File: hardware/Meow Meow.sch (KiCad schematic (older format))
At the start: 28 parts, among them P1 D, P10 A, P11 W, P12 MOUSE_LEFT, P13 CONN_01X06, P14 CONN_01X06, P2 SPACE, P3 KEY_RIGHT_ARROW, P4 SWD, P5 KEY_LEFT_ARROW, P6 KEY_DOWN_ARROW, P7 KEY_UP_ARROW, P8 S, P9 USB_Micro, SW1 SW_Push, U1 ATSAMD21G18A-AU, U2 AP2114-3.3K

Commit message: Add pin 5v
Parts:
- removed P13, P14: CONN_01X06, Pines:61000618321, symbol CONN_01X06
- added P? (x2): CONN_01X07, symbol CONN_01X07
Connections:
- wire segments 97 -> 101
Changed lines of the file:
@@
 Title "Meow Meow"
 Date "2018-05-16"
-Rev "0.7"
+Rev "0.8"
 Comp "Electronic Cats"
 Comment1 "Andres Sabas"
@@
 	8745 3600 8745 3570
 $Comp
-L CONN_01X06 P13
-U 1 1 5B1DE3E8
-P 9090 6010
-F 0 "P13" H 9090 6360 50  0000 C CNN
-F 1 "CONN_01X06" V 9190 6010 50  0000 C CNN
-F 2 "Pines:61000618321" H 9090 6010 50  0001 C CNN
-F 3 "" H 9090 6010 50  0000 C CNN
-	1    9090 6010
-	1    0    0    -1
-$EndComp
-$Comp
-L CONN_01X06 P14
-U 1 1 5B1DE934
-P 9570 5980
-F 0 "P14" H 9570 6330 50  0000 C CNN
-F 1 "CONN_01X06" V 9670 5980 50  0000 C CNN
-F 2 "Pines:61000618321" H 9570 5980 50  0001 C CNN
-F 3 "" H 9570 5980 50  0000 C CNN
-	1    9570 5980
+L CONN_01X07 P?
+U 1 1 5B26BBAC
+P 9090 6060
+F 0 "P?" H 9090 6460 50  0000 C CNN
+F 1 "CONN_01X07" V 9190 6060 50  0000 C CNN
+F 2 "" H 9090 6060 50  0000 C CNN
+F 3 "" H 9090 6060 50  0000 C CNN
+	1    9090 6060
+	1    0    0    -1
+$EndComp
+$Comp
+L CONN_01X07 P?
+U 1 1 5B26BCF3
+P 9570 6030
+F 0 "P?" H 9570 6430 50  0000 C CNN
+F 1 "CONN_01X07" V 9670 6030 50  0000 C CNN
+F 2 "" H 9570 6030 50  0000 C CNN
+F 3 "" H 9570 6030 50  0000 C CNN
+	1    9570 6030
 	-1   0    0    1
 $EndComp
+Wire Wire Line
+	8355 6360 8890 6360
+$Comp
+L VCC #PWR?
+U 1 1 5B26C1A1
+P 8355 6340
+F 0 "#PWR?" H 8355 6190 50  0001 C CNN
+F 1 "VCC" H 8355 6490 50  0000 C CNN
+F 2 "" H 8355 6340 50  0000 C CNN
+F 3 "" H 8355 6340 50  0000 C CNN
+	1    8355 6340
+	1    0    0    -1
+$EndComp
+Wire Wire Line
+	8355 6360 8355 6340
+Wire Wire Line
+	9770 6330 9815 6330
+Wire Wire Line
+	9815 6330 9815 6230
+Connection ~ 9815 6230
 $EndSCHEMATC

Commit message: connector 6 pin
se quito 3V
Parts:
- removed P? (x2): CONN_01X07, symbol CONN_01X07
- added J? (x2): Conn_02x03_Top_Bottom, symbol Conn_02x03_Top_Bottom
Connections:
- wire segments 101 -> 97
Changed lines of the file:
@@
 Text Notes 7805 5625 0    60   ~ 0
 PIN EXTRAS
-Text Label 9870 5730 0    60   ~ 0
+Text Label 10025 6130 0    60   ~ 0
 I2S_SCK
-Text Label 9875 5830 0    60   ~ 0
+Text Label 10025 6030 0    60   ~ 0
 I2S_D1/X7
-Text Label 9875 5930 0    60   ~ 0
+Text Label 10020 5930 0    60   ~ 0
 TX/X2
-Text Label 9875 6030 0    60   ~ 0
+Text Label 9340 6130 2    60   ~ 0
 RX/X3
-Text Label 8780 5760 2    60   ~ 0
-MOSI
-Text Label 8780 5860 2    60   ~ 0
+Text Label 8105 6025 2    60   ~ 0
 MISO
-Text Label 8780 5960 2    60   ~ 0
+Text Label 8105 6125 2    60   ~ 0
 SCK
-Text Label 9875 6130 0    60   ~ 0
+Text Label 9335 6030 2    60   ~ 0
 CS
-Text Label 8785 6060 2    60   ~ 0
+Text Label 8820 5925 0    60   ~ 0
 SDA
-Text Label 8785 6160 2    60   ~ 0
+Text Label 8815 6025 0    60   ~ 0
 SCL
 $Comp
 L GND #PWR019
 U 1 1 5AFF5159
-P 9890 6230
-F 0 "#PWR019" H 9890 5980 50  0001 C CNN
-F 1 "GND" H 9890 6080 50  0000 C CNN
-F 2 "" H 9890 6230 50  0000 C CNN
-F 3 "" H 9890 6230 50  0000 C CNN
-	1    9890 6230
-	1    0    0    -1
-$EndComp
-$Comp
-L +3.3V #PWR020
-U 1 1 5AFF522D
-P 8500 6260
-F 0 "#PWR020" H 8500 6110 50  0001 C CNN
-F 1 "+3.3V" H 8500 6400 50  0000 C CNN
-F 2 "" H 8500 6260 50  0000 C CNN
-F 3 "" H 8500 6260 50  0000 C CNN
-	1    8500 6260
-	1    0    0    -1
+P 9335 5930
+F 0 "#PWR019" H 9335 5680 50  0001 C CNN
+F 1 "GND" H 9335 5780 50  0000 C CNN
+F 2 "" H 9335 5930 50  0000 C CNN
+F 3 "" H 9335 5930 50  0000 C CNN
+	1    9335 5930
+	-1   0    0    1
 $EndComp
 $Comp
@@
 	3895 1655 4210 1655
 Wire Wire Line
-	3990 1955 3990 1565
-Wire Wire Line
-	3895 1955 3990 1955
+	3990 1565 3990 1955
+Wire Wire Line
+	3990 1955 3895 1955
 Wire Wire Line
 	3945 2285 3945 2340
@@
 Connection ~ 4025 4655
 Wire Wire Line
-	3895 4655 4025 4655
+	4025 4655 3895 4655
 Connection ~ 4025 4555
 Wire Wire Line
-	3895 4555 4025 4555
+	4025 4555 3895 4555
 Wire Wire Line
 	4025 4355 4025 4740
@@
 Connection ~ 9605 1290
 Wire Wire Line
-	9605 1355 9605 1290
+	9605 1290 9605 1355
 Connection ~ 9370 1290
 Wire Wire Line
@@
 	7590 1290 7590 1175
 Wire Wire Line
-	8315 1290 7590 1290
+	7590 1290 8315 1290
 Wire Wire Line
 	9810 5100 9810 5325
@@
 	1590 1655 1590 1675
 Wire Wire Line
-	8890 6160 8785 6160
-Wire Wire Line
-	8890 6060 8785 6060
-Wire Wire Line
-	8890 5960 8780 5960
-Wire Wire Line
-	8890 5860 8780 5860
-Wire Wire Line
-	8890 5760 8780 5760
-Wire Wire Line
-	9770 6130 9875 6130
-Wire Wire Line
-	9770 6030 9875 6030
-Wire Wire Line
-	9770 5930 9875 5930
-Wire Wire Line
-	9770 5830 9875 5830
-Wire Wire Line
-	9770 5730 9870 5730
-Wire Wire Line
-	8500 6260 8890 6260
-Wire Wire Line
-	9770 6230 9890 6230
-Wire Wire Line
 	9100 3285 8970 3285
 Wire Wire Line
@@
 	8745 3600 8745 3570
 $Comp
-L CONN_01X07 P?
-U 1 1 5B26BBAC
-P 9090 6060
-F 0 "P?" H 9090 6460 50  0000 C CNN
-F 1 "CONN_01X07" V 9190 6060 50  0000 C CNN
-F 2 "" H 9090 6060 50  0000 C CNN
-F 3 "" H 9090 6060 50  0000 C CNN
-	1    9090 6060
-	1    0    0    -1
-$EndComp
-$Comp
-L CONN_01X07 P?
-U 1 1 5B26BCF3
-P 9570 6030
-F 0 "P?" H 9570 6430 50  0000 C CNN
-F 1 "CONN_01X07" V 9670 6030 50  0000 C CNN
-F 2 "" H 9570 6030 50  0000 C CNN
-F 3 "" H 9570 6030 50  0000 C CNN
-	1    9570 6030
-	-1   0    0    1
-$EndComp
-Wire Wire Line
-	8355 6360 8890 6360
+L Conn_02x03_Top_Bottom J?
+U 1 1 5B57974D
+P 9640 6030
+F 0 "J?" H 9690 6230 50  0000 C CNN
+F 1 "Conn_02x03_Top_Bottom" H 9690 5830 50  0000 C CNN
+F 2 "" H 9640 6030 50  0001 C CNN
+F 3 "" H 9640 6030 50  0001 C CNN
+	1    9640 6030
+	1    0    0    -1
+$EndComp
+Text Label 8105 5925 2    60   ~ 0
+MOSI
+$Comp
+L Conn_02x03_Top_Bottom J?
+U 1 1 5B57970D
+P 8390 6025
+F 0 "J?" H 8440 6225 50  0000 C CNN
+F 1 "Conn_02x03_Top_Bottom" H 8330 5840 50  0000 C CNN
+F 2 "" H 8390 6025 50  0001 C CNN
+F 3 "" H 8390 6025 50  0001 C CNN
+	1    8390 6025
+	1    0    0    -1
+$EndComp
+Wire Wire Line
+	8105 5925 8190 5925
+Wire Wire Line
+	8105 6025 8190 6025
+Wire Wire Line
+	8105 6125 8190 6125
 $Comp
 L VCC #PWR?
 U 1 1 5B26C1A1
-P 8355 6340
-F 0 "#PWR?" H 8355 6190 50  0001 C CNN
-F 1 "VCC" H 8355 6490 50  0000 C CNN
-F 2 "" H 8355 6340 50  0000 C CNN
-F 3 "" H 8355 6340 50  0000 C CNN
-	1    8355 6340
-	1    0    0    -1
-$EndComp
-Wire Wire Line
-	8355 6360 8355 6340
-Wire Wire Line
-	9770 6330 9815 6330
-Wire Wire Line
-	9815 6330 9815 6230
-Connection ~ 9815 6230
+P 8870 6125
+F 0 "#PWR?" H 8870 5975 50  0001 C CNN
+F 1 "VCC" H 8870 6265 50  0000 C CNN
+F 2 "" H 8870 6125 50  0000 C CNN
+F 3 "" H 8870 6125 50  0000 C CNN
+	1    8870 6125
+	-1   0    0    1
+$EndComp
+Wire Wire Line
+	8690 5925 8820 5925
+Wire Wire Line
+	8690 6025 8815 6025
+Wire Wire Line
+	8870 6125 8690 6125
+Wire Wire Line
+	9940 5930 10020 5930
+Wire Wire Line
+	9940 6030 10025 6030
+Wire Wire Line
+	9940 6130 10025 6130
+Wire Wire Line
+	9440 5930 9335 5930
+Wire Wire Line
+	9440 6030 9335 6030
+Wire Wire Line
+	9440 6130 9340 6130
 $EndSCHEMATC

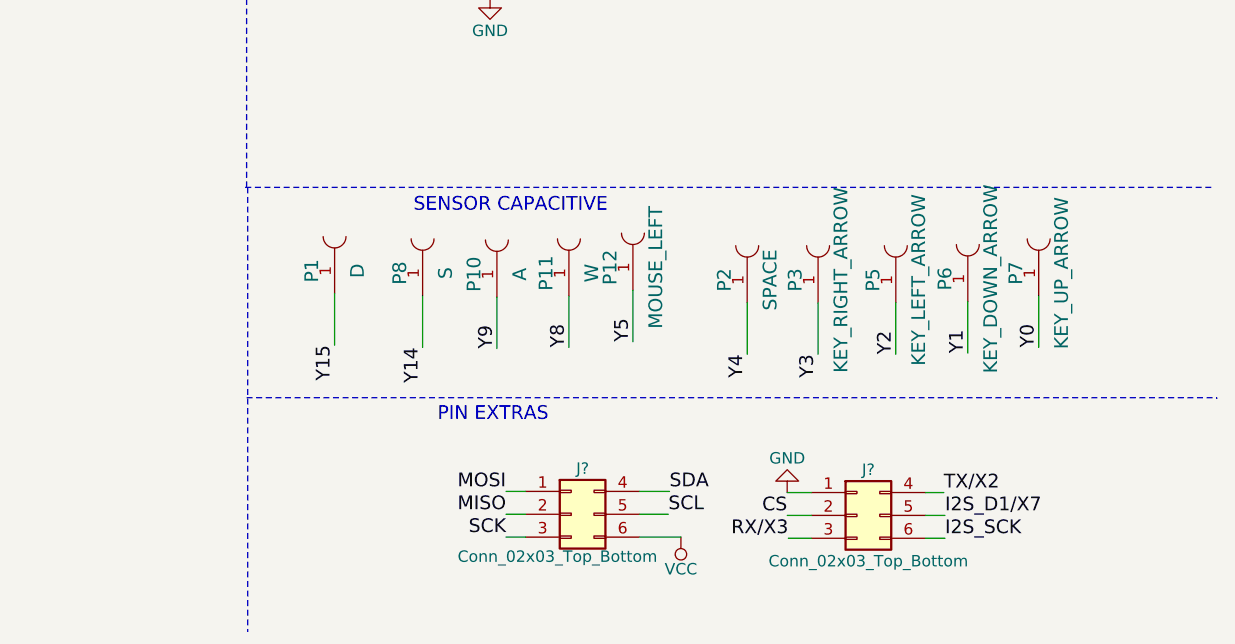
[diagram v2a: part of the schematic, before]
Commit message: SENSOR CAPACITIVE
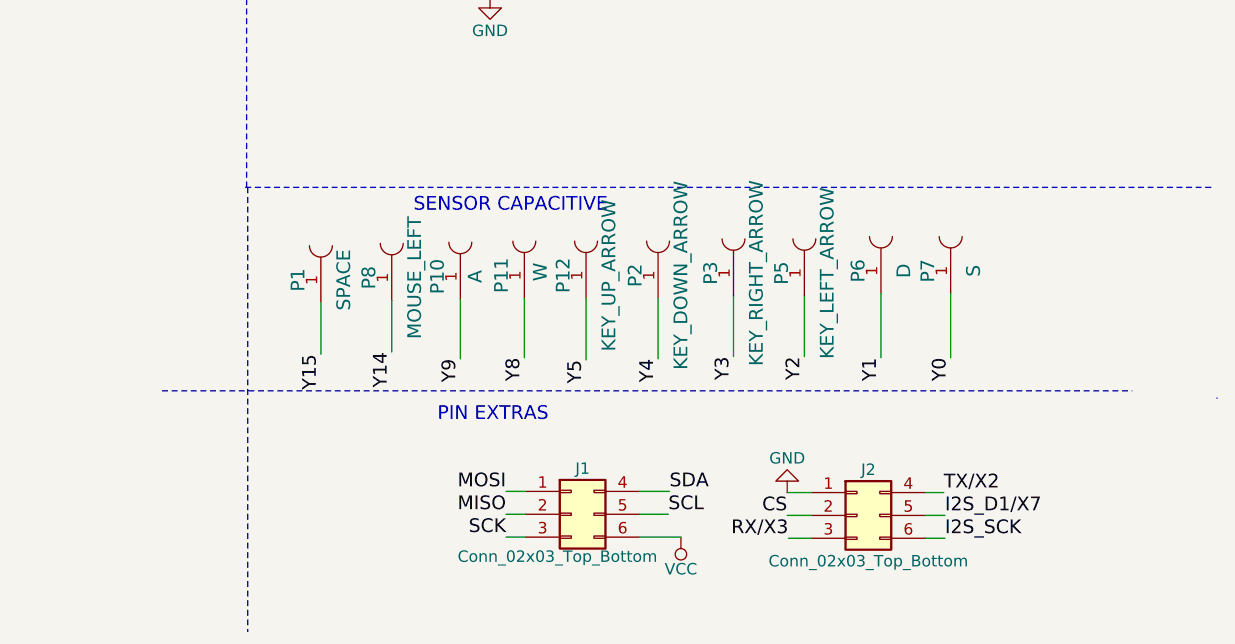
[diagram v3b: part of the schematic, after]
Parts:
- P1: value D -> SPACE
- P12: value MOUSE_LEFT -> KEY_UP_ARROW
- P2: value SPACE -> KEY_DOWN_ARROW
- P6: value KEY_DOWN_ARROW -> D
- P7: value KEY_UP_ARROW -> S
- P8: value S -> MOUSE_LEFT
- gave numbers to parts that had none: 2
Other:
- moved on the sheet: P1, P10, P11, P12, P2, P3, P5, P6, P7, P8
